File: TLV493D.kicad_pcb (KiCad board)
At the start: 2 copper layers, 11.7 x 22.6 mm, 10 parts, among them J1 Conn_01x04_Female, U1 TLV493D

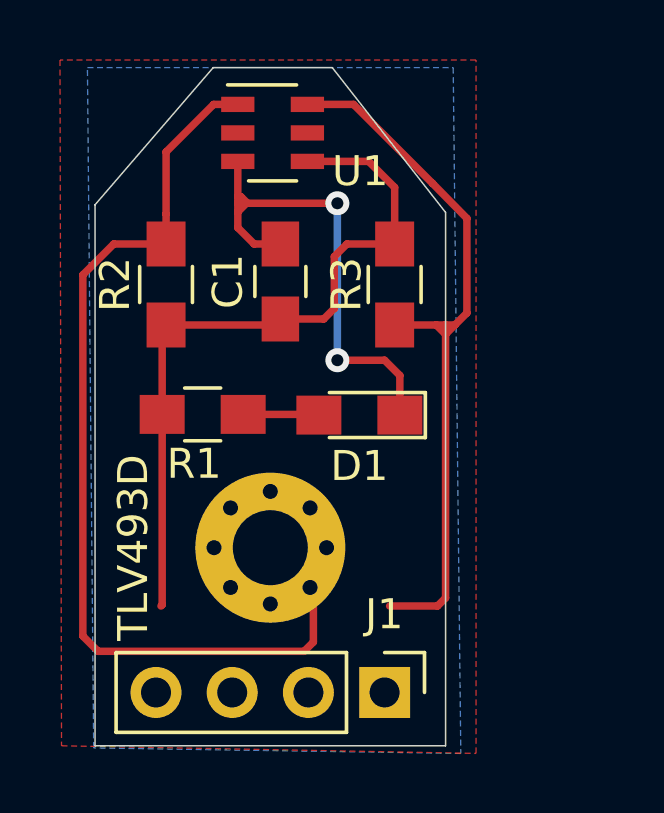
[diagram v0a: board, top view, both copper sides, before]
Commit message: re routeo
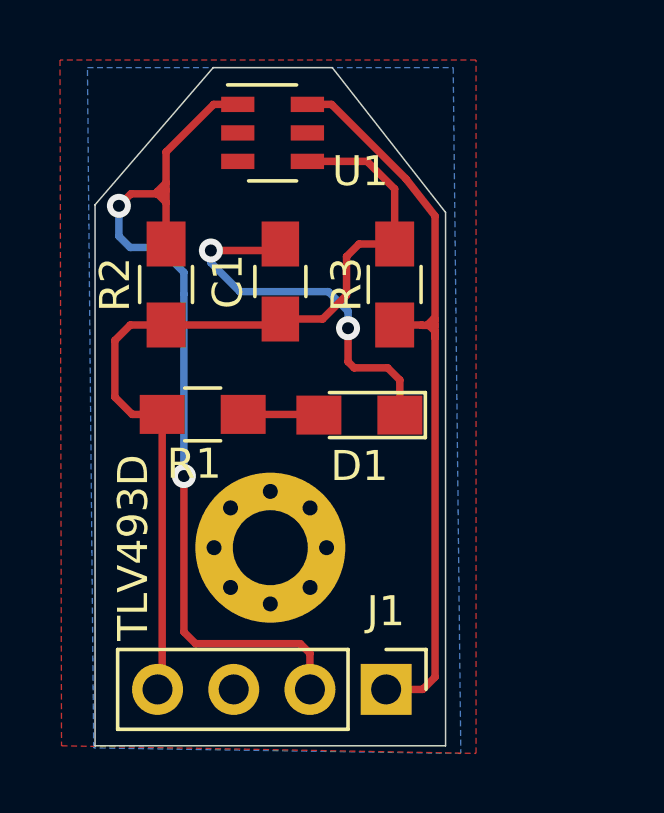
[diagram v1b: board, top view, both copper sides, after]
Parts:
- moved J1 0.11 mm to (157.8, 118.8)
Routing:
- net VCC: track 24.3 -> 29.5 mm
- net GND: track 16.9 -> 12.9 mm
- net /SDA: track 24.6 -> 25.3 mm
- net /SCL: track 30.6 -> 30.2 mm, vias 0 -> 2

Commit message: VCC,GND,SCL,SDA
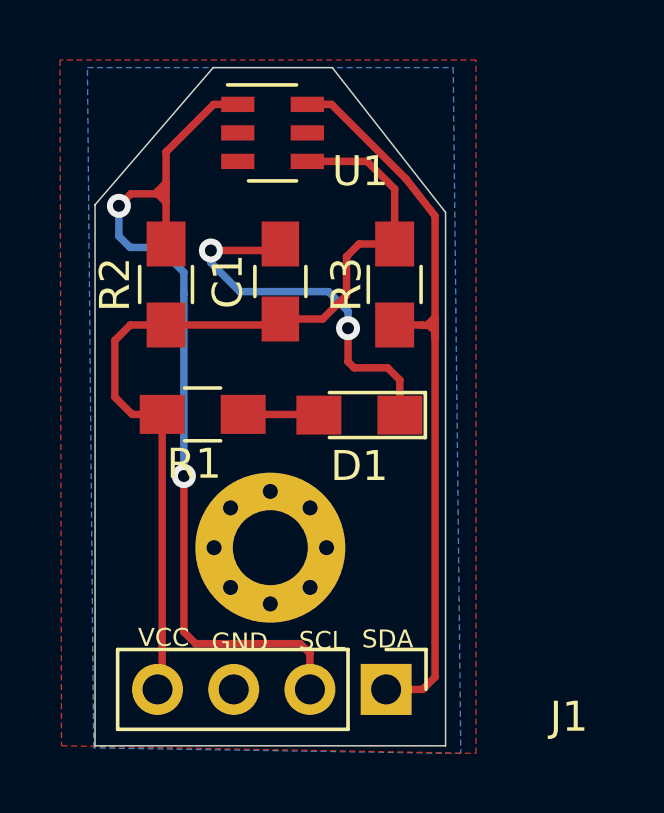
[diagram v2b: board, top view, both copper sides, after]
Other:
- board text added: "GND"
- board text added: "SCL"
- board text added: "SDA"
- board text added: "VCC"
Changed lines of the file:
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@@
   (general
     (thickness 1.6)
-    (drawings 10)
+    (drawings 14)
     (tracks 78)
     (zones 0)
@@
     (mod_text_size 1 1)
     (mod_text_width 0.15)
-    (pad_size 1.11 0.51)
-    (pad_drill 0)
+    (pad_size 1.7 1.7)
+    (pad_drill 1)
     (pad_to_mask_clearance 0.051)
     (solder_mask_min_width 0.25)
@@
       (effects (font (size 1 1) (thickness 0.15)) (justify mirror))
     )
-    (fp_text value OSHW-Logo2_7.3x6mm_SilkScreen (at 0.75 0) (layer B.Fab) hide
+    (fp_text value OSHW-Logo2_7.3x6mm_SilkScreen (at 0.75 0) (layer F.Fab) hide
       (effects (font (size 1 1) (thickness 0.15)) (justify mirror))
     )
@@
     (descr "Through hole straight pin header, 1x04, 2.54mm pitch, single row")
     (tags "Through hole pin header THT 1x04 2.54mm single row")
-    (fp_text reference J1 (at -2.6044 0.0136 180) (layer F.SilkS)
+    (fp_text reference J1 (at 0.9144 -6.096 180) (layer F.SilkS)
       (effects (font (size 1 1) (thickness 0.15)))
     )
@@
     )
   )
+  (gr_text VCC (at 150.368 117.0432) (layer F.SilkS)
+    (effects (font (size 0.6 0.6) (thickness 0.15)))
+  )
+  (gr_text GND (at 152.908 117.1956) (layer F.SilkS)
+    (effects (font (size 0.6 0.6) (thickness 0.15)))
+  )
+  (gr_text SCL (at 155.6512 117.1448) (layer F.SilkS)
+    (effects (font (size 0.6 0.6) (thickness 0.15)))
+  )
+  (gr_text SDA (at 157.8356 117.094) (layer F.SilkS)
+    (effects (font (size 0.6 0.6) (thickness 0.15)))
+  )
   (gr_text TLV493D (at 153.924 117.348) (layer B.SilkS)
     (effects (font (size 1 1) (thickness 0.25)) (justify mirror))
   )
-  (gr_text TLV493D (at 149.352 114.046 90) (layer F.SilkS)
+  (gr_text TLV493D (at 149.352 114.046 90) (layer F.Fab)
     (effects (font (size 1 1) (thickness 0.25)))
   )
